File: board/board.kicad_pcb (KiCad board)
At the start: 2 copper layers, 92 x 75.8 mm, 68 parts, among them J2 Conn_01x01, J3 Conn_01x01, J3 Conn_01x25_Socket, J4 Conn_01x01, J4 Conn_01x25_Socket, J5 Conn_01x01, J5 PJ-320B, J6 Screw_Terminal_01x02, J7 Screw_Terminal_01x02, J8 Screw_Terminal_01x02

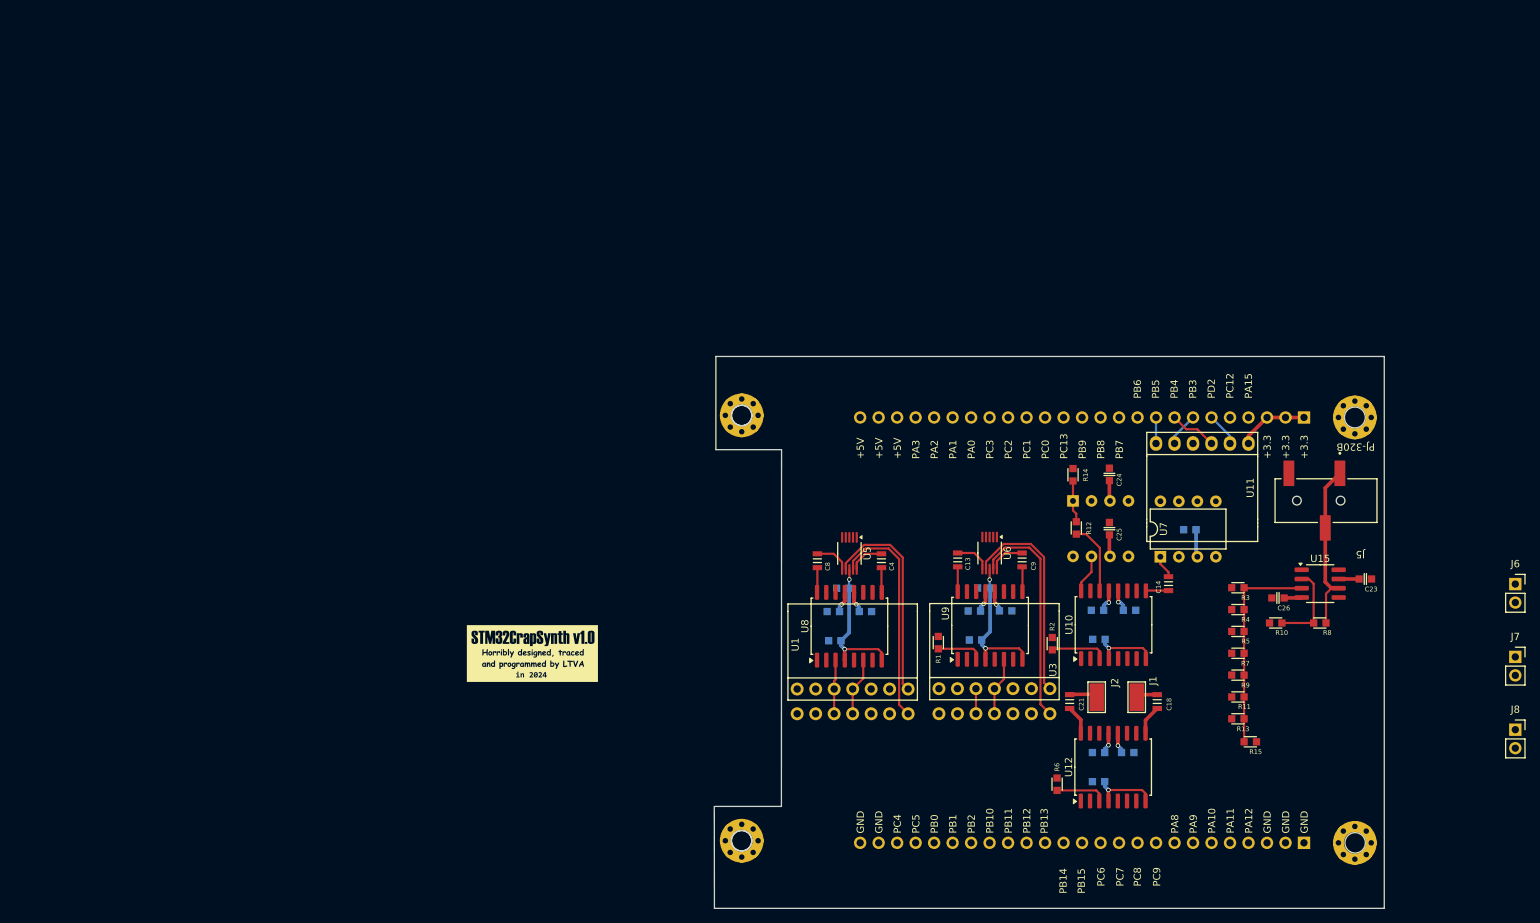
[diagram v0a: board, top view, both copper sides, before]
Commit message: more board rework, UART & SPI init
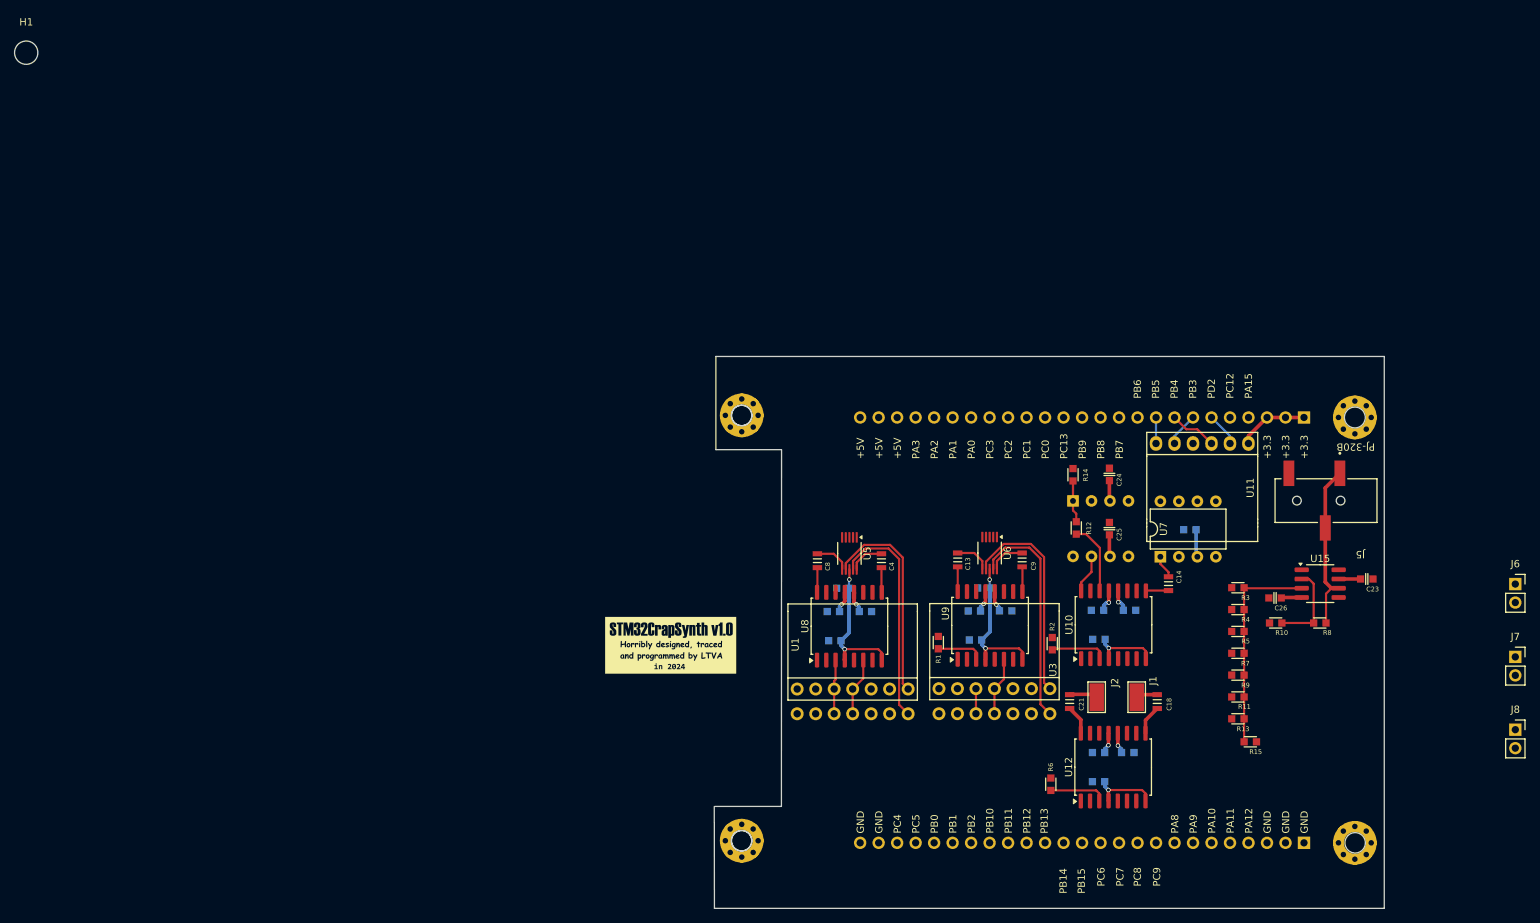
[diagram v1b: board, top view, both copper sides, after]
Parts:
- added H1: MountingHole, MountingHole:MountingHole_3.2mm_M3, F.Cu at (3.48, 3.48)
- moved G*** 19.0 mm to (92.0, 84.9)
- moved R6 0.87 mm to (144.2, 104.0)
- moved C26 0.40 mm to (175.0, 78.4)
- moved C23 0.20 mm to (187.6, 75.8)
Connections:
- J3 pad 11: ZCEN_2 -> /PC7
- J3 pad 12: ZCEN_1 -> ATTEN_CS
- J3 pad 14: /PB14/adc4_in4 -> ZCEN_DAC
- J3 pad 16: /PB12/adc4_in3 -> ZCEN_2
- J3 pad 17: /PB11 -> CS_AD9833_4
- J3 pad 18: /PB10 -> CS_AD9833_3
- J3 pad 19: /PB2 -> ZCEN_1
- J3 pad 22: /PC5/adc2_in11 -> CS_AD9833_1
- J3 pad 23: /PC4/adc2_in5 -> CS_AD9833_2
- J3 pad 6: CS_AD9833_3 -> /PA10
- J3 pad 7: CS_AD9833_2 -> /PA9
- J3 pad 9: ZCEN_DAC -> /PC9
- J4 pad 14: MUX_SEL_3 -> NOISE_CLK_SEL
- J4 pad 15: MUX_SEL_4 -> NOISE_CS
- J4 pad 16: NOISE_CLK_SEL -> /PC1
- J4 pad 18: MUX_SEL_1 -> MUX_SEL_4
- J4 pad 19: MUX_SEL_2 -> MUX_SEL_3
- J4 pad 21: ATTEN_CS -> MUX_SEL_1
- J4 pad 22: CS_AD9833_1 -> MUX_SEL_2
- J4 pad 4: NOISE_CS -> /PA15
- J4 pad 5: CS_AD9833_4 -> /PC12
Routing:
- net Analog_data_out3: track 7.00 -> 7.86 mm
